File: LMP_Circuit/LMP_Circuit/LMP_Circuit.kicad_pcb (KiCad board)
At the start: 2 copper layers, 126.5 x 91.7 mm, 6 parts, among them K1 SANYOU_SRD_Form_C, U2 DQD2_Single

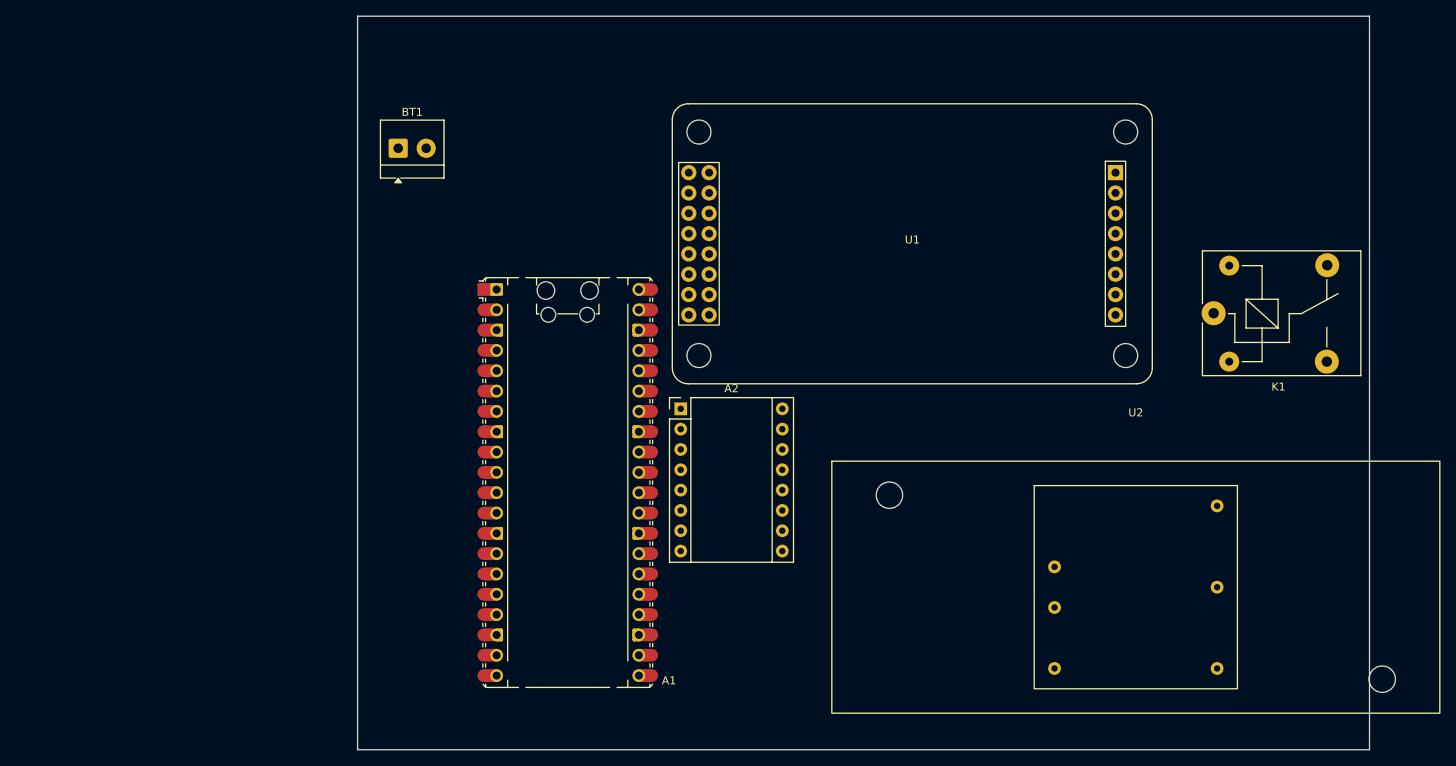
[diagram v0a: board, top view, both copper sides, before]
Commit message: initial layout created.
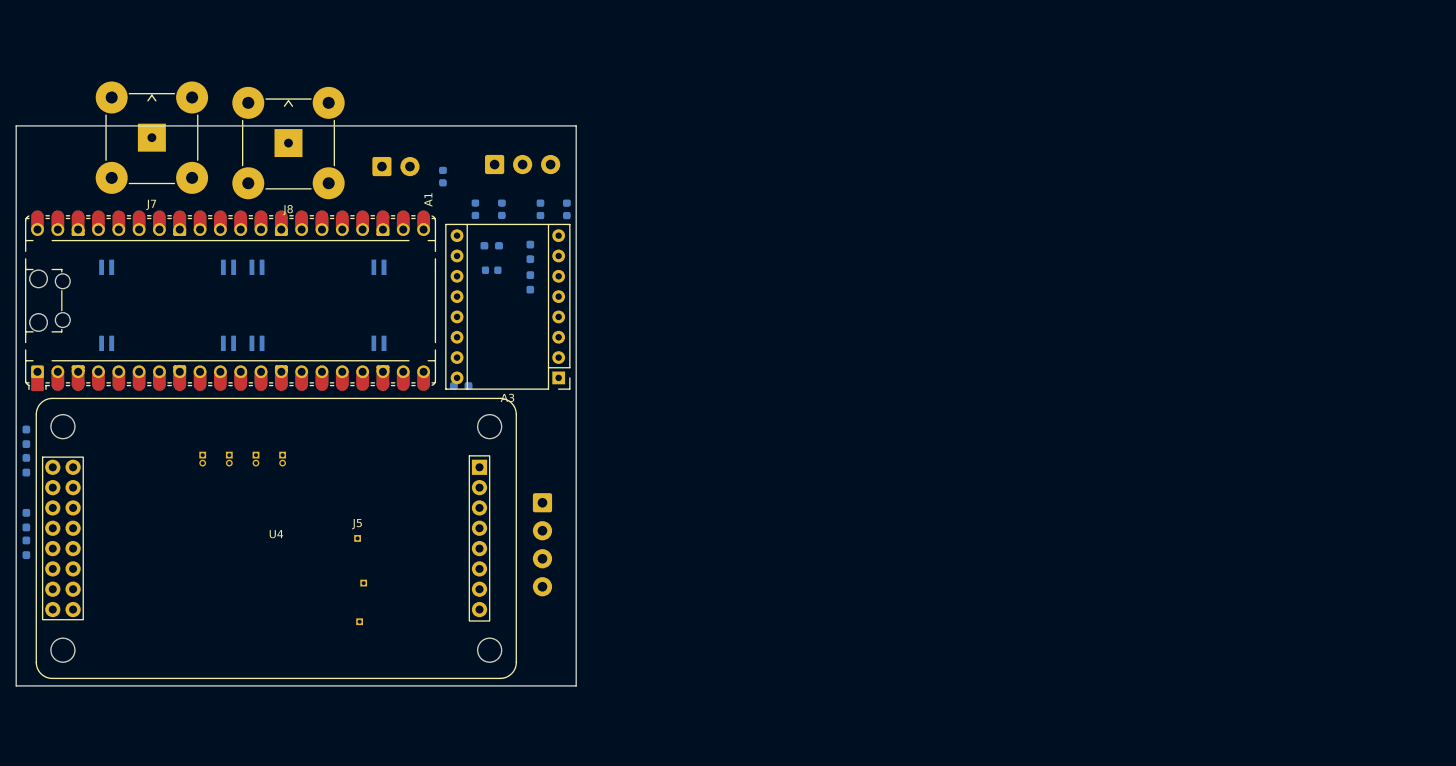
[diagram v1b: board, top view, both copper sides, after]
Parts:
- removed A2: Pololu_Breakout_A4988, Module:Pololu_Breakout-16_15.2x20.3mm
- removed BT1: Battery, TerminalBlock_4Ucon:TerminalBlock_4Ucon_1x02_P3.50mm_Horizontal
- removed K1: SANYOU_SRD_Form_C, Relay_THT:Relay_SPDT_SANYOU_SRD_Series_Form_C
- removed U2: DQD2_Single, External/Custom Parts:DQD20
- added A3: Pololu_Breakout_A4988, Module:Pololu_Breakout-16_15.2x20.3mm, F.Cu at (125.0, 102.9)
- added C1: 100nf, Capacitor_SMD:C_0603_1608Metric, B.Cu at (110.5, 77.7)
- added C2: 10uf, Capacitor_SMD:C_0603_1608Metric, B.Cu at (114.6, 81.8)
- added C3: 100n, Capacitor_SMD:C_0603_1608Metric, B.Cu at (117.9, 81.8)
- added C4: 10uf, Capacitor_SMD:C_0603_1608Metric, B.Cu at (122.7, 81.8)
- added C5: 100nf, Capacitor_SMD:C_0603_1608Metric, B.Cu at (126.0, 81.8)
- added C6: 10uf, Capacitor_SMD:C_0603_1608Metric, B.Cu at (116.6, 89.4)
- added J1: SCLK, Connector_PinHeader_1.00mm:PinHeader_1x02_P1.00mm_Vertical, B.Cu at (90.5, 112.5)
- added J10: RX, Connector_PinHeader_1.00mm:PinHeader_1x01_P1.00mm_Vertical, B.Cu at (100.1, 133.3)
- added J11: Stepper_Terminals, TerminalBlock_4Ucon:TerminalBlock_4Ucon_1x04_P3.50mm_Horizontal, B.Cu at (122.9, 118.5)
- added J12: ISO_Power_Terminal, TerminalBlock_4Ucon:TerminalBlock_4Ucon_1x02_P3.50mm_Horizontal, B.Cu at (102.9, 76.5)
- added J2: MOSI, Connector_PinHeader_1.00mm:PinHeader_1x02_P1.00mm_Vertical, B.Cu at (87.1, 112.5)
- added J3: MISO, Connector_PinHeader_1.00mm:PinHeader_1x02_P1.00mm_Vertical, B.Cu at (83.8, 112.5)
- added J4: MISO, Connector_PinHeader_1.00mm:PinHeader_1x02_P1.00mm_Vertical, B.Cu at (80.5, 112.5)
- added J5: Relay_Trig, Connector_PinHeader_1.00mm:PinHeader_1x01_P1.00mm_Vertical, B.Cu at (99.8, 122.9)
- added J6: Power Terminal, TerminalBlock_4Ucon:TerminalBlock_4Ucon_1x03_P3.50mm_Horizontal, B.Cu at (117.0, 76.2)
- added J7: Electrode+, Connector_Coaxial:BNC_TEConnectivity_1478035_Horizontal, F.Cu at (74.1, 72.8)
- added J8: Electrode-, Connector_Coaxial:BNC_TEConnectivity_1478035_Horizontal, F.Cu at (91.2, 73.5)
- added J9: TX, Connector_PinHeader_1.00mm:PinHeader_1x01_P1.00mm_Vertical, B.Cu at (100.6, 128.5)
- added R10: 1k, Resistor_SMD:R_0603_1608Metric_Pad0.98x0.95mm_HandSolder, B.Cu at (121.4, 90.9)
- added R11: 1k, Resistor_SMD:R_0603_1608Metric_Pad0.98x0.95mm_HandSolder, B.Cu at (112.8, 103.9)
- added R3: 5M, Resistor_SMD:R_0603_1608Metric_Pad0.98x0.95mm_HandSolder, B.Cu at (116.6, 86.4)
- added R5: 23.57k, Resistor_SMD:R_0603_1608Metric_Pad0.98x0.95mm_HandSolder, B.Cu at (58.4, 110.2)
- added R6: 3.84k, Resistor_SMD:R_0603_1608Metric_Pad0.98x0.95mm_HandSolder, B.Cu at (58.4, 113.8)
- added R7: 23.57k, Resistor_SMD:R_0603_1608Metric_Pad0.98x0.95mm_HandSolder, B.Cu at (58.4, 120.7)
- added R8: 3.84k, Resistor_SMD:R_0603_1608Metric_Pad0.98x0.95mm_HandSolder, B.Cu at (58.4, 124.1)
- added R9: 1M, Resistor_SMD:R_0603_1608Metric_Pad0.98x0.95mm_HandSolder, B.Cu at (121.4, 87.1)
- added U3: ISO124U/1K, External/Custom Parts:ISO124U, B.Cu at (94.9, 93.8)
- added U4: ADS1256, External/Custom Parts:ADS1256, F.Cu at (89.7, 122.9)
- U1: value ~ -> ISO124U/1K; footprint External/Custom Parts:ADS1256 -> External/Custom Parts:ISO124U; moved to B.Cu
- moved U1 93.4 mm to (76.1, 93.8), turned to 90 degrees
- moved A1 47.9 mm to (83.9, 93.2), turned to 90 degrees
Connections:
- A1 pad 1: /Relay_Trigger -> /TX
- A1 pad 2: unconnected-(A1-GPIO1-Pad2) -> /RX
- A1 pad 20: unconnected-(A1-GPIO15-Pad20) -> /PhotoMos
- A1 pad 27: unconnected-(A1-GPIO21-Pad27) -> Net-(A1-GPIO21)
- A1 pad 29: unconnected-(A1-GPIO22-Pad29) -> Net-(A1-GPIO22)
- A1 pad 36: unconnected-(A1-3V3-Pad36) -> +3.3V
- A1 pad 4: unconnected-(A1-GPIO2-Pad4) -> /Relay_Trigger
- U1 pad 1: +5V -> Probe_28V
- U1 pad 13: unconnected-(U1-A4-Pad13) -> Net-(U1-VOUT)
- U1 pad 14: unconnected-(U1-A5-Pad14) -> GND
- U1 pad 15: unconnected-(U1-A6-Pad15) -> 28V
- U1 pad 16: unconnected-(U1-A7-Pad16) -> GND
- U1 pad 2: GND -> GND1
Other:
- board size 126.5 x 91.7 mm -> 70 x 70 mm
